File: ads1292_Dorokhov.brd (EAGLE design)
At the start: 40 x 30 mm, 61 parts, among them IC1 TPS77001, Q1 BSS84, U1 LIS344AL

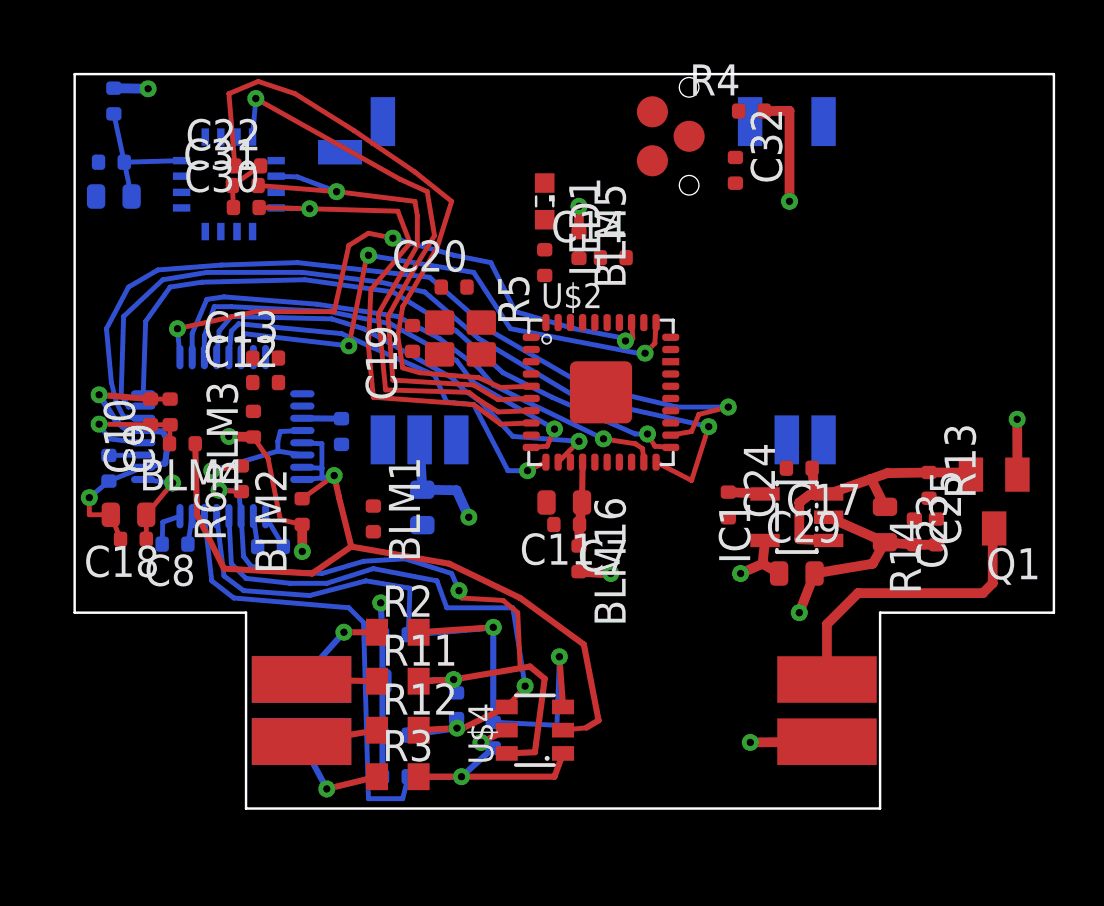
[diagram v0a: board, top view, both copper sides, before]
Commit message: Rev.2.0
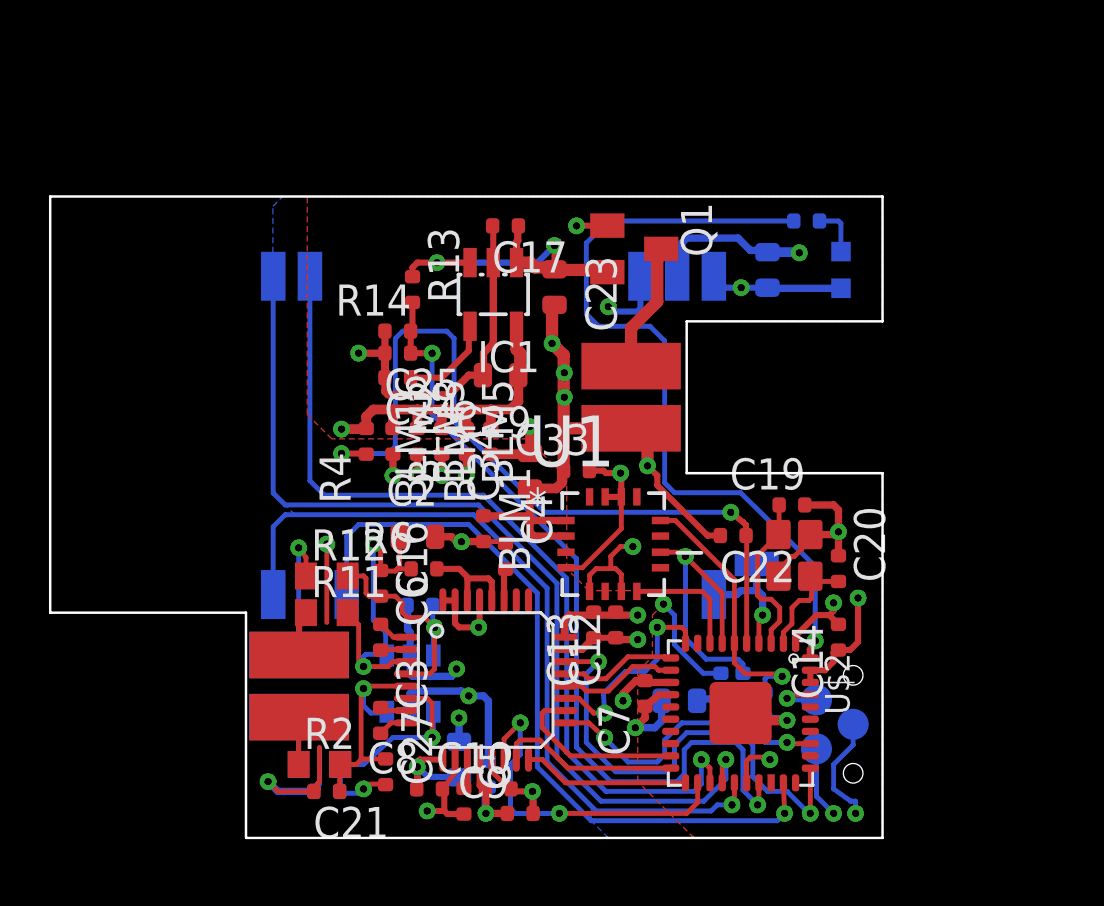
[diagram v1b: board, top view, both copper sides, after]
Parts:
- moved C30 29.4 mm to (28.2, 4.20), flipped to the bottom, turned to 90 degrees
- moved C31 28.8 mm to (27.3, 5.00), flipped to the bottom, turned to 90 degrees
- moved JP3 24.9 mm to (30.8, 3.44), flipped to the bottom, turned to 90 degrees
- moved C22 24.9 mm to (26.9, 11.2), turned to 180 degrees
- moved R14 23.5 mm to (13.2, 19.5), turned to 0 degrees
- moved C33 22.8 mm to (20.5, 13.8), flipped to the top, turned to 0 degrees
- moved R13 22.6 mm to (13.8, 21.2)
- moved C25 22.3 mm to (13.2, 18.6), turned to 180 degrees
- moved C9 21.8 mm to (18.2, -0.20), turned to 0 degrees
- moved U1 21.5 mm to (22.0, 10.8), flipped to the top, turned to 0 degrees
- moved C32 21.1 mm to (26.4, 5.00), flipped to the bottom, turned to 90 degrees
- moved C10 20.9 mm to (17.3, 0.80), turned to 0 degrees
- moved BLM6 20.7 mm to (17.0, 15.0), flipped to the top
- moved R4 20.7 mm to (11.9, 15.0), turned to 90 degrees
- moved C34 20.4 mm to (18.6, 13.8), flipped to the top, turned to 90 degrees
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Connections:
- removed net N$29: C16.P$3, C2.P$1, R11.2, R6.P$3, U$1.P$3, U$4.6
- new net N$15: C1.P$3, C16.P$4, R12.2, U$1.P$4, U$4.6
- net ACC_X: now also U$2.6; no longer U$2.8
- net ACC_Z: now also U$2.8; no longer U$2.6
- net AGND: no longer LED1.C
- net GND: now also LED1.C
- net N$21: now also R2.1; no longer R12.1
- net N$22: now also R12.1; no longer R2.1
- net N$23: now also C16.P$3, C2.P$1, R11.2, R6.P$3, U$1.P$3; no longer C1.P$3, C16.P$4, R12.2, U$1.P$4
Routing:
- net GND: track 19.3 -> 147.9 mm, vias 3 -> 14
- net AGND: track 23.2 -> 79.9 mm, vias 4 -> 8
- net RX: track 0.00 -> 39.1 mm, vias 0 -> 1
- net BT_RST: track 0.00 -> 37.4 mm, vias 0 -> 2
- net TX: track 0.00 -> 36.4 mm, vias 0 -> 1
- net BATT_ADC: track 0.00 -> 33.7 mm, vias 0 -> 2
- net N$13: track 0.00 -> 32.7 mm, vias 0 -> 1
- net N$29: track 32.2 -> 0.00 mm, vias 3 -> 0
- net BT_PROG: track 0.00 -> 32.1 mm, vias 0 -> 1
- net BT_CON_STAT: track 0.00 -> 31.0 mm, vias 0 -> 1
- net ADS_RESET: track 34.4 -> 7.61 mm, vias 1 -> 0
- net N$12: track 0.00 -> 24.2 mm, vias 0 -> 2
- net RST: track 26.3 -> 50.2 mm, vias 0 -> 3
- net N$2: track 3.43 -> 25.6 mm, vias 0 -> 2
- net CLCSEL: track 35.5 -> 14.2 mm, vias 1 -> 2
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- added copper zone on layer 1, net GND
- added copper zone on layer 15, net GND
- added copper zone on layer 16, net GND
- added copper zone on layer 2, net GND
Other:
- board size 40 x 30 mm -> 34 x 26.2 mm

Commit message: REV_3.0
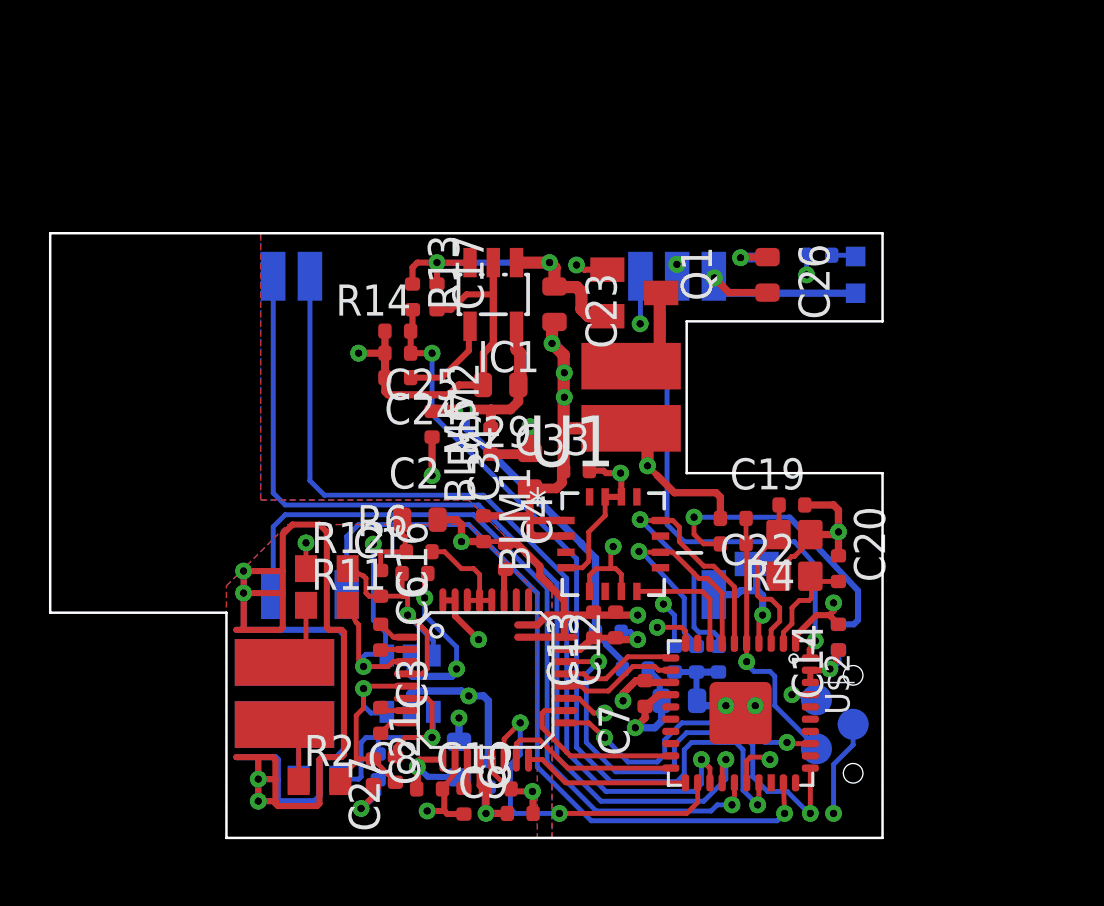
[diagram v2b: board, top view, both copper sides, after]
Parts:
- moved BLM5 17.2 mm to (31.2, 7.00), flipped to the bottom
- moved R4 15.6 mm to (26.9, 10.8), turned to 180 degrees
- moved BLM16 12.2 mm to (22.9, 5.70), flipped to the bottom, turned to 0 degrees
- moved BLM3 11.0 mm to (21.8, 7.20), flipped to the bottom, turned to 180 degrees
- moved C17 4.03 mm to (14.8, 20.9), turned to 270 degrees
- moved C30 2.69 mm to (26.3, 6.10)
- moved C15 2.33 mm to (12.4, 1.70), turned to 270 degrees
- moved C31 2.20 mm to (25.4, 6.10)
- moved C32 2.20 mm to (24.5, 6.10)
- moved C21 2.06 mm to (12.2, 1.50), turned to 270 degrees
- moved Q1 1.80 mm to (22.9, 21.1)
- moved BLM2 1.75 mm to (14.6, 15.7)
- moved R5 1.49 mm to (30.4, 22.6)
- moved C1 1.32 mm to (13.9, 9.60), flipped to the top
- moved R6 0.73 mm to (14.1, 10.5)
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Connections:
- removed net N$18: R6.P$4, U$1.P$28, U$1.P$30
- new net N$27: R6.P$4, U$1.P$28, U$1.P$29, U$1.P$30
- net +3V3: no longer U$1.P$29
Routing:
- net AGND: track 79.9 -> 136.1 mm, vias 8 -> 12
- net RST: track 50.2 -> 11.0 mm, vias 3 -> 1
- net N$12: track 24.2 -> 3.16 mm, vias 2 -> 1
- net +3,3D: track 46.3 -> 66.2 mm, vias 2 -> 4
- net N$2: track 25.6 -> 5.84 mm, vias 2 -> 1
- net N$1: track 18.8 -> 4.61 mm, vias 2 -> 1
- net GND: track 147.9 -> 156.3 mm, vias 14 -> 15
- net BT_RST: track 37.4 -> 29.1 mm
- net N$13: track 32.7 -> 27.3 mm, vias 1 -> 3
- net N$27: track 0.00 -> 4.39 mm
- net N$18: track 4.16 -> 0.00 mm
- net ACC_X: track 10.9 -> 14.5 mm
- net N$22: track 5.71 -> 8.06 mm, vias 1 -> 2
- net ACC_Z: track 9.89 -> 7.58 mm
- net N$15: track 10.0 -> 11.5 mm
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- added copper zone on layer 2, net +3,3D
- added copper zone on layer 2, net +3V3
- added copper zone on layer 1, net AGND
- added copper zone on layer 15, net AGND
- added copper zone on layer 16, net AGND
- removed copper zone on layer 2, net GND
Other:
- board size 34 x 26.2 mm -> 34 x 24.7 mm
